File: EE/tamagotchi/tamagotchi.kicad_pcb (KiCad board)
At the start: 2 copper layers, 6.2 x 1.8 mm, 42 parts, among them J7 TAG_CONNECT, P1 USB_C_Plug_USB2.0, SW2 TL1260BQRBLK, U2 STM32G031G8Ux

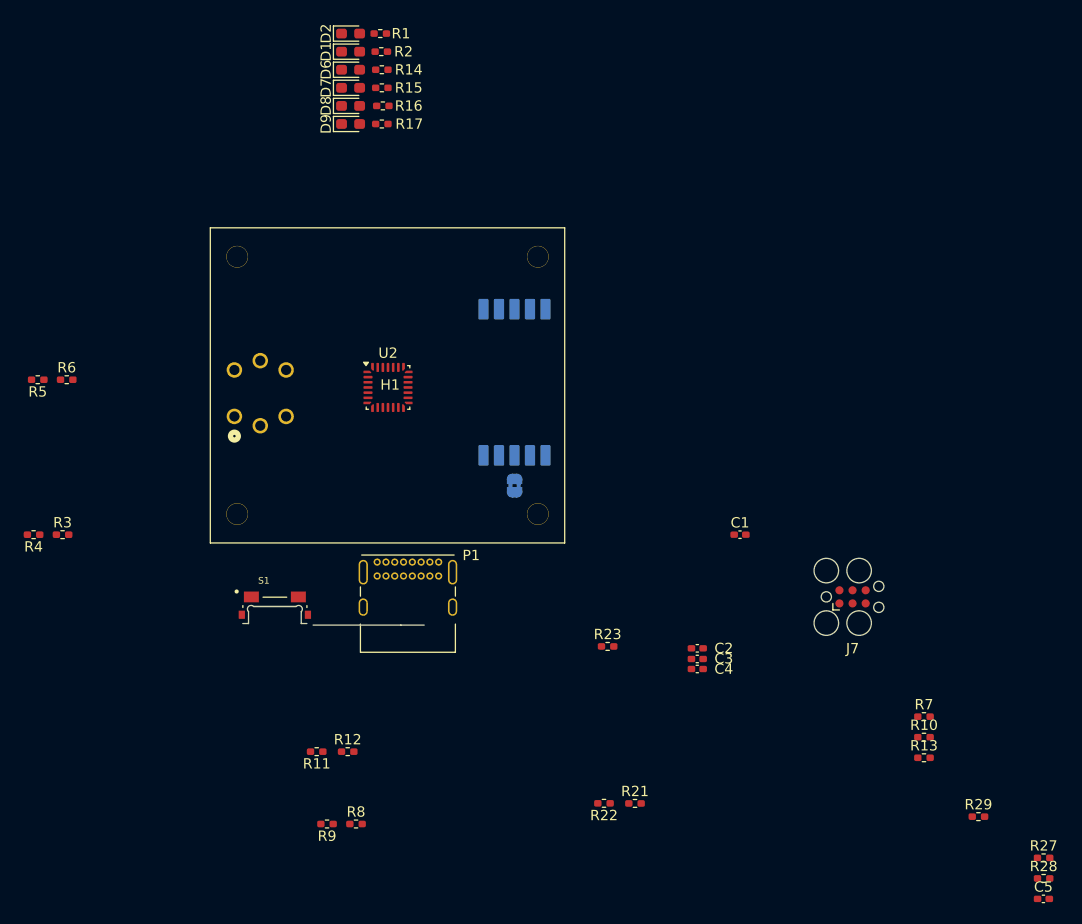
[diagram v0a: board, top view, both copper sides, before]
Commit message: Basic Placement Complete
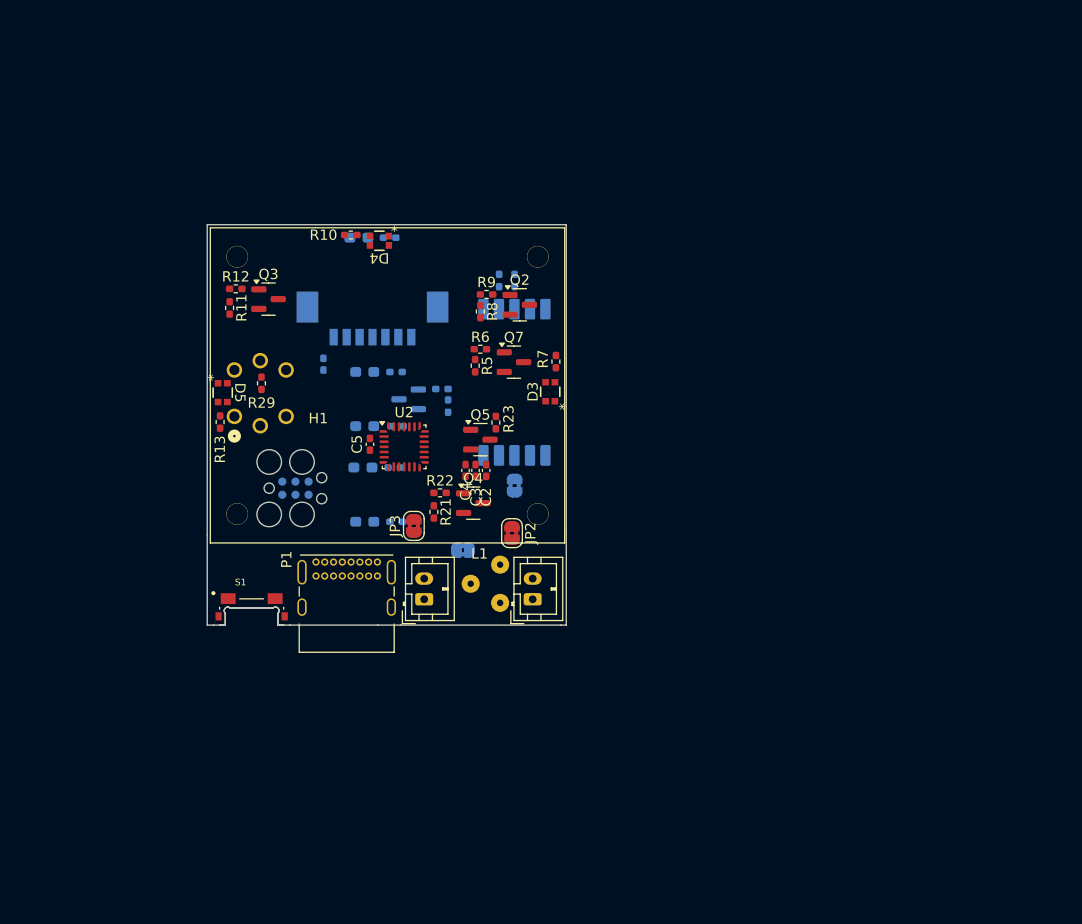
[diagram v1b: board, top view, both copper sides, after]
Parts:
- removed D2: LED, LED_SMD:LED_0603_1608Metric_Pad1.05x0.95mm_HandSolder
- removed R1: R, Resistor_SMD:R_0402_1005Metric_Pad0.72x0.64mm_HandSolder
- added BATTERY: Conn_01x02_Male, Connector_JST:JST_PH_B2B-PH-K_1x02_P2.00mm_Vertical, F.Cu at (167.5, 107.3)
- added D3: LED_BRGY, Library:EAST1616RGYA0_EVE, F.Cu at (169.2, 87.2)
- added D4: LED_BRGY, Library:EAST1616RGYA0_EVE, F.Cu at (152.7, 72.6)
- added D5: LED_BRGY, Library:EAST1616RGYA0_EVE, F.Cu at (137.5, 87.2)
- added J3: Conn_01x07, Library:MOLEX_532610771, B.Cu at (152.0, 79.5)
- added JP2: SolderJumper_2_Bridged, Jumper:SolderJumper-2_P1.3mm_Bridged2Bar_RoundedPad1.0x1.5mm, F.Cu at (165.5, 100.9)
- added JP3: SolderJumper_2_Bridged, Jumper:SolderJumper-2_P1.3mm_Bridged2Bar_RoundedPad1.0x1.5mm, F.Cu at (156.0, 100.1)
- added JP4: SolderJumper_2_Bridged, Jumper:SolderJumper-2_P1.3mm_Bridged2Bar_RoundedPad1.0x1.5mm, B.Cu at (160.8, 102.5)
- added L1: ~, Library:UT Transformer, F.Cu at (161.5, 105.8)
- added Q1: Q_NMOS_GSD, Package_TO_SOT_SMD:SOT-23, B.Cu at (155.5, 87.9)
- added Q2: Q_NMOS_GSD, Package_TO_SOT_SMD:SOT-23, F.Cu at (166.2, 78.8)
- added Q3: Q_NMOS_GSD, Package_TO_SOT_SMD:SOT-23, F.Cu at (141.9, 78.2)
- added Q4: Q_NMOS_GSD, Package_TO_SOT_SMD:SOT-23, F.Cu at (161.8, 98.0)
- added Q5: Q_PMOS_GSD, Package_TO_SOT_SMD:SOT-23, F.Cu at (162.4, 91.8)
- added Q7: Q_NMOS_GSD, Package_TO_SOT_SMD:SOT-23, F.Cu at (165.7, 84.3)
- added UT: Conn_01x02_Male, Connector_JST:JST_PH_B2B-PH-K_1x02_P2.00mm_Vertical, F.Cu at (157.0, 107.2)
- C1, D1, D6, D7, D8, D9, J7, R14, R15, R16, R17, R2, R27, R28, R3, R4: moved to B.Cu
- moved R29 81.1 mm to (141.2, 86.3), turned to 90 degrees
- moved C5 78.6 mm to (151.8, 92.2), turned to -90 degrees
- moved R28 78.3 mm to (164.2, 76.4), turned to -90 degrees
- moved R27 75.8 mm to (165.8, 76.4), turned to -90 degrees
- moved R13 75.5 mm to (137.2, 90.1), turned to 90 degrees
- moved R10 73.7 mm to (149.9, 72.0)
- moved J7 54.9 mm to (144.5, 96.5)
- moved R9 53.5 mm to (163.0, 77.8), turned to 0 degrees
- moved R8 51.0 mm to (162.4, 79.4), turned to -90 degrees
- moved R7 49.5 mm to (169.8, 84.2), turned to -90 degrees
- moved R12 46.1 mm to (138.8, 77.2)
- moved R11 43.8 mm to (138.2, 79.1), turned to -90 degrees
- moved C1 43.6 mm to (147.2, 84.5), turned to -90 degrees
- moved R5 42.4 mm to (161.9, 84.6), turned to -90 degrees
- moved R4 42.0 mm to (158.7, 86.9)
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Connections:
- JP1 pad 1: /Power/VBAT_BRIDGED -> Net-(J8-Pin_1)
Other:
- board size 6.2 x 1.8 mm -> 34.8 x 38.8 mm
